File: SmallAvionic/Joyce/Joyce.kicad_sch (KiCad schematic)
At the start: 1 part, among them U1 STM32F103C8Tx

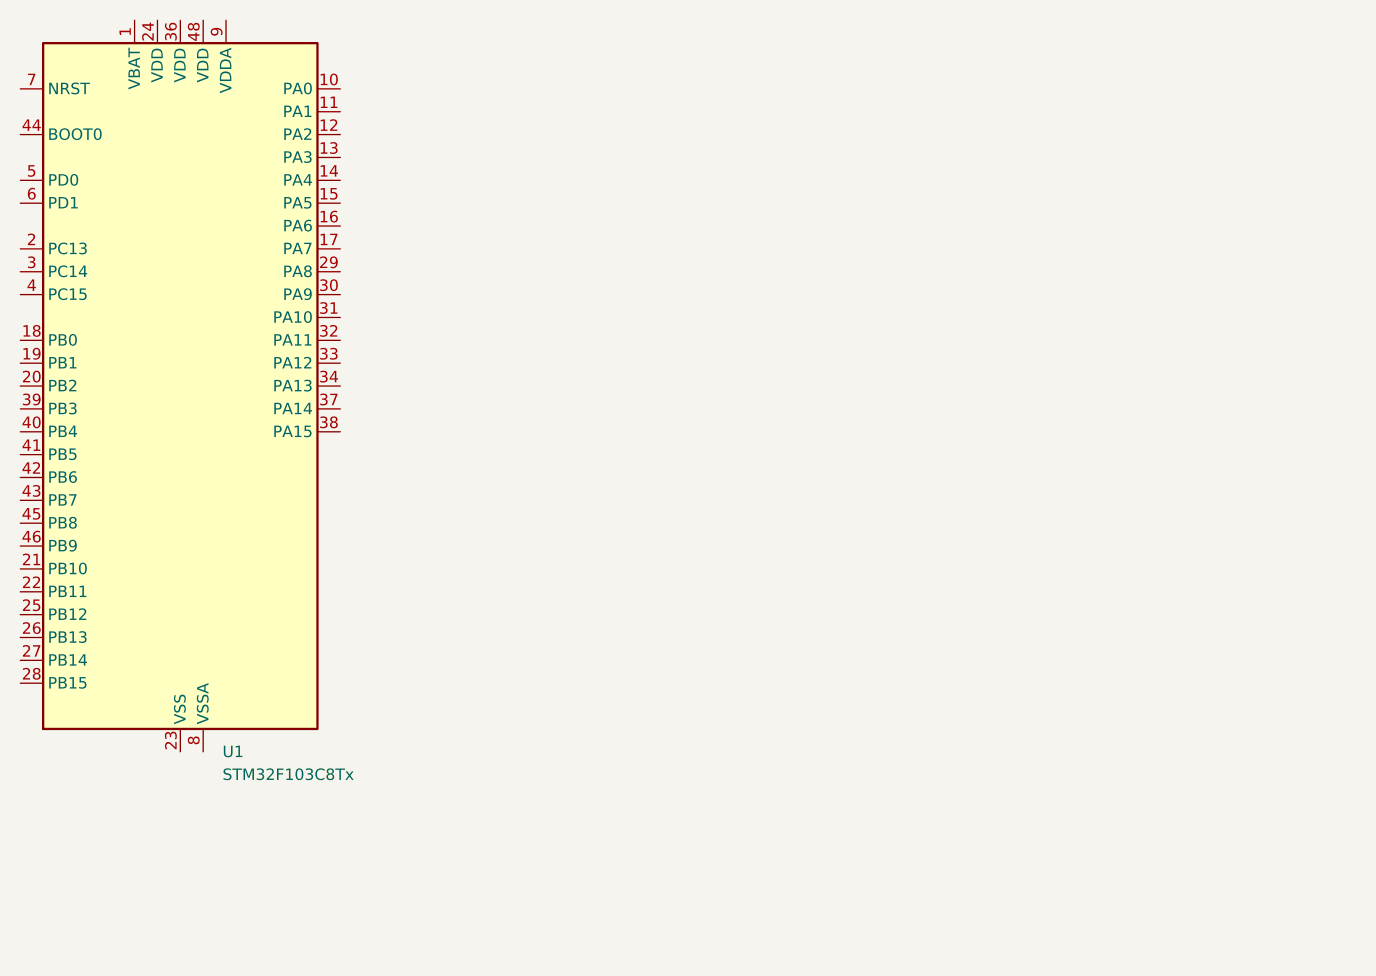
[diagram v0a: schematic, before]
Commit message: Joyce push 1/22
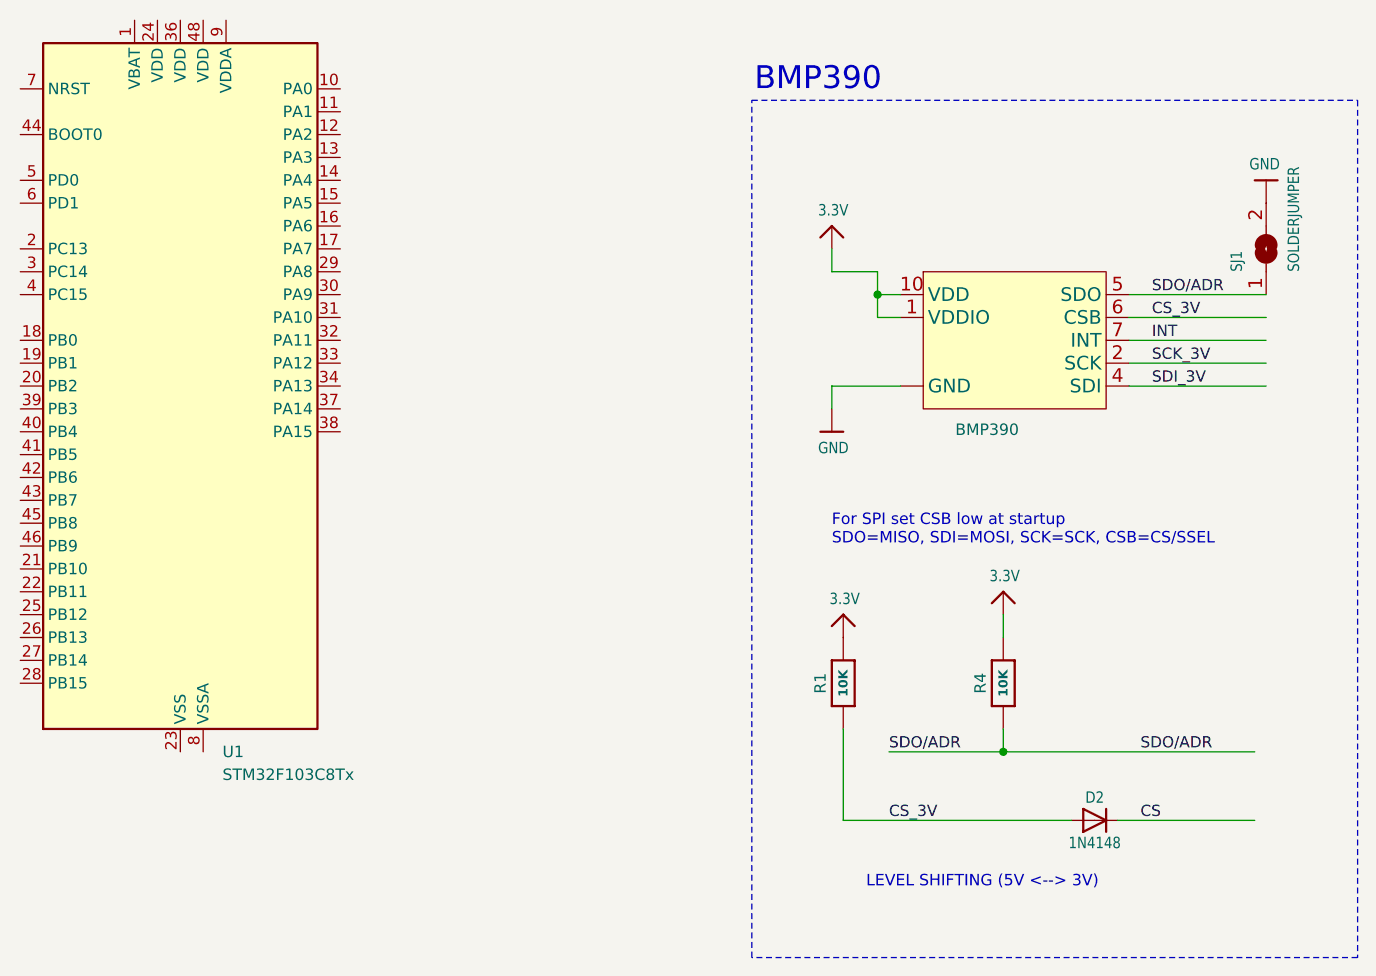
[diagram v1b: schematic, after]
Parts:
- added D2: 1N4148, Adafruit BMP390:SOD-323, symbol Adafruit BMP390-eagle-import:microbuilder_DIODESOD-323
- added IC1: BMP390, Adafruit BMP390:BMP388, symbol Adafruit BMP390-eagle-import:microbuilder_BMP388
- added R1, R4: 10K, Adafruit BMP390:0603-NO, symbol Adafruit BMP390-eagle-import:microbuilder_RESISTOR_0603_NOOUT
- added SJ1: SOLDERJUMPER, Adafruit BMP390:SOLDERJUMPER_ARROW_NOPASTE, symbol Adafruit BMP390-eagle-import:microbuilder_SOLDERJUMPER
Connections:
- new net 3.3V: IC1.1 (VDDIO), IC1.10 (VDD), R1.2, R4.2
- new net CS: D2.C
- new net CS_3V: D2.A, IC1.6 (CSB), R1.1
- new net GND: IC1.3 (GND), IC1.8 (GND), IC1.9 (GND), SJ1.2
- new net INT: IC1.7 (INT)
- new net SCK_3V: IC1.2 (SCK)
- new net SDI_3V: IC1.4 (SDI)
- new net SDO/ADR: IC1.5 (SDO), R4.1, SJ1.1
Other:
- note added: "BMP390"
- note added: "For SPI set CSB low at startup SDO=MISO, SDI=MOSI, SCK=SCK, CSB=CS/SSEL"
- note added: "LEVEL SHIFTING (5V <--> 3V)"
